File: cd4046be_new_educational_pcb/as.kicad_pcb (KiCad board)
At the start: 2 copper layers, 43.5 x 29.5 mm, 9 parts, among them IC1 CD4046BE, J1 Conn_01x02_Socket, J2 Conn_01x08_Socket, J3 Conn_01x08_Socket, J4 Conn_01x02_Socket, J5 Conn_01x02_Socket, J6 Conn_01x02_Socket, J7 Conn_01x02_Socket, J8 Conn_01x02_Socket

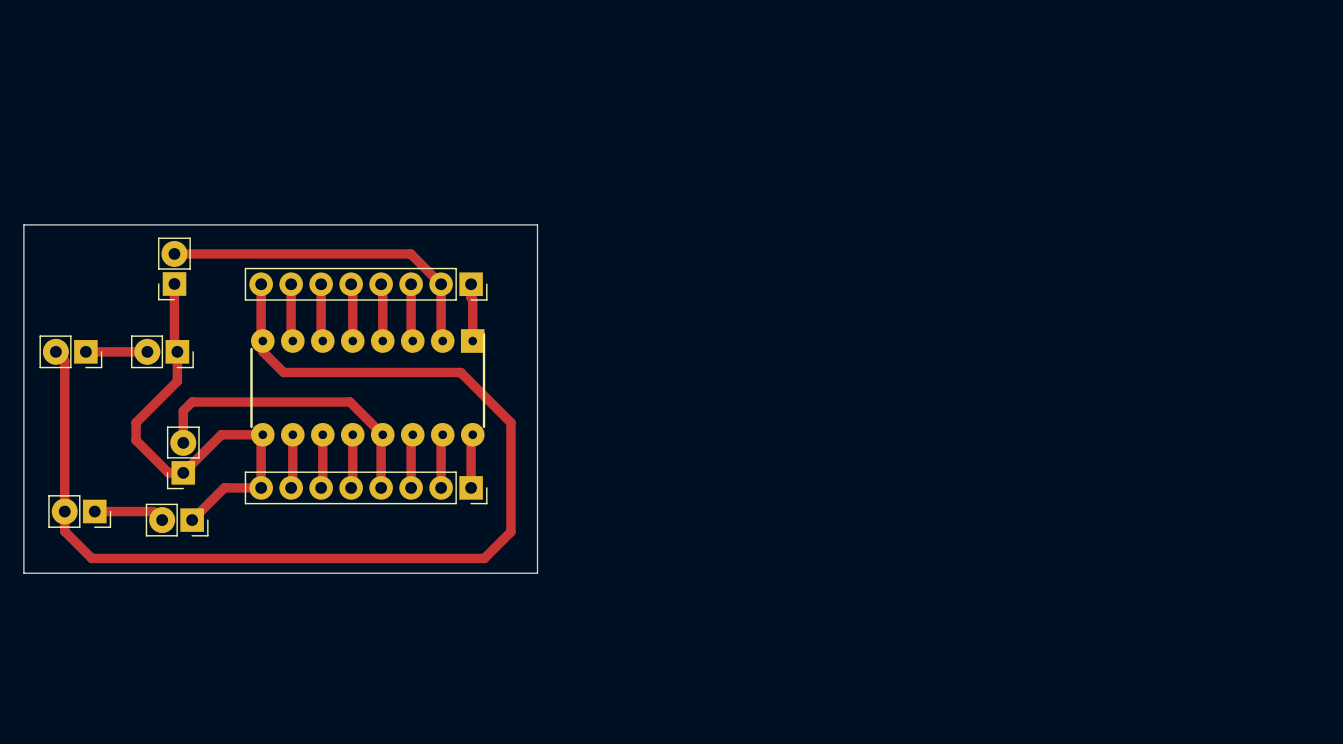
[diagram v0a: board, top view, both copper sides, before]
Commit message: a
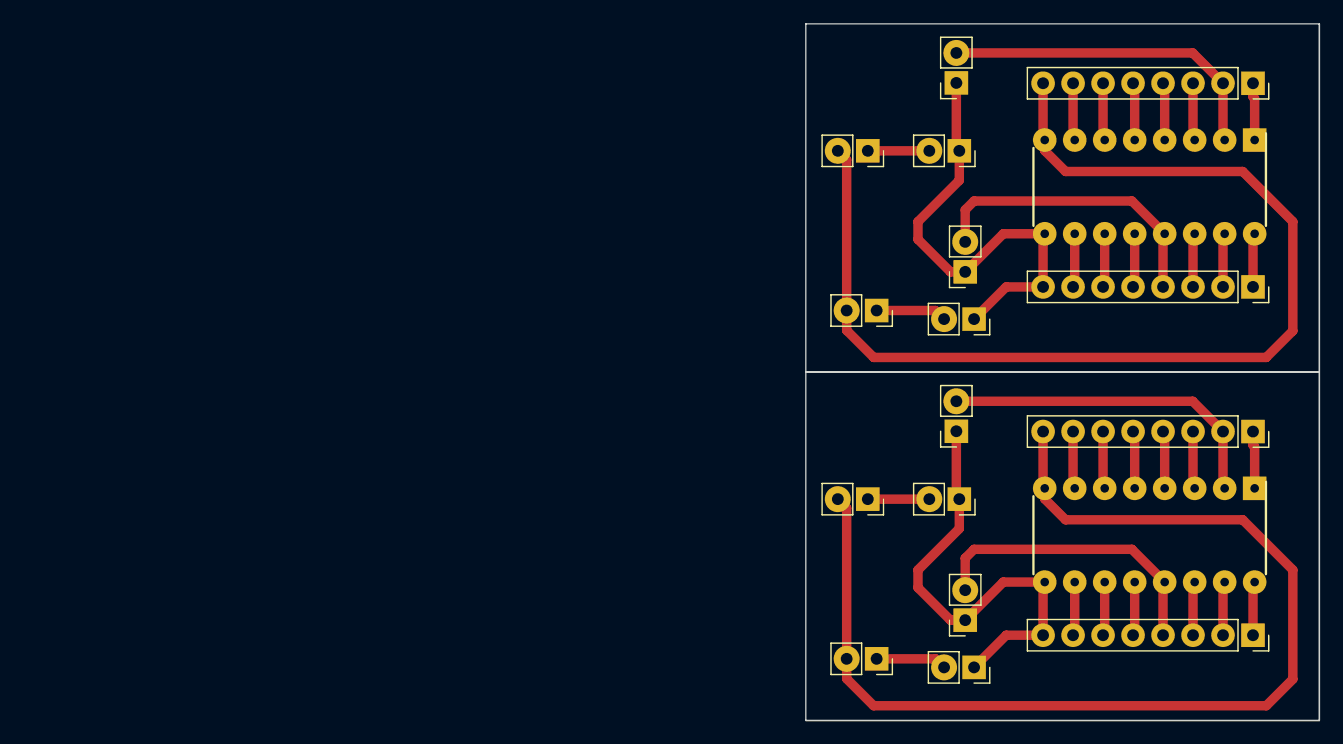
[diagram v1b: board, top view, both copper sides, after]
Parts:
- added IC1: CD4046BE, KiCad:DIP794W53P254L1930H508Q16N, F.Cu at (220.3, 107.5)
- added J1: Conn_01x02_Socket, Connector_PinSocket_2.54mm:PinSocket_1x02_P2.54mm_Vertical, F.Cu at (204.0, 98.7)
- added J2: Conn_01x08_Socket, Connector_PinSocket_2.54mm:PinSocket_1x08_P2.54mm_Vertical, F.Cu at (229.1, 98.8)
- added J3: Conn_01x08_Socket, Connector_PinSocket_2.54mm:PinSocket_1x08_P2.54mm_Vertical, F.Cu at (229.1, 116.0)
- added J4: Conn_01x02_Socket, Connector_PinSocket_2.54mm:PinSocket_1x02_P2.54mm_Vertical, F.Cu at (204.2, 104.5)
- added J5: Conn_01x02_Socket, Connector_PinSocket_2.54mm:PinSocket_1x02_P2.54mm_Vertical, F.Cu at (196.5, 104.5)
- added J6: Conn_01x02_Socket, Connector_PinSocket_2.54mm:PinSocket_1x02_P2.54mm_Vertical, F.Cu at (204.7, 114.7)
- added J7: Conn_01x02_Socket, Connector_PinSocket_2.54mm:PinSocket_1x02_P2.54mm_Vertical, F.Cu at (197.2, 118.0)
- added J8: Conn_01x02_Socket, Connector_PinSocket_2.54mm:PinSocket_1x02_P2.54mm_Vertical, F.Cu at (205.5, 118.7)
- moved IC1 68.4 mm to (220.3, 78.0)
- moved J1 68.4 mm to (204.0, 69.2)
- moved J2 68.4 mm to (229.1, 69.2)
- moved J3 68.4 mm to (229.1, 86.5)
- moved J4 68.4 mm to (204.2, 75.0)
- moved J5 68.4 mm to (196.5, 75.0)
- moved J6 68.4 mm to (204.7, 85.2)
- moved J7 68.4 mm to (197.2, 88.5)
- moved J8 68.4 mm to (205.5, 89.2)
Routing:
- net GND: track 93.7 -> 187.4 mm
- net /VCO_IN: track 40.7 -> 81.4 mm
- net /PC1: track 28.5 -> 57.0 mm
- net /PC2: track 25.6 -> 51.2 mm
- net Net-(J7-Pin_1): track 6.01 -> 12.0 mm
- net Net-(J4-Pin_2): track 5.21 -> 10.4 mm
- net Net-(IC1-PHASE_PULSES): track 4.87 -> 9.74 mm
- net Net-(IC1-INHIBIT): track 4.87 -> 9.74 mm
- net Net-(IC1-VCO_OUT): track 4.87 -> 9.74 mm
- net Net-(IC1-CI(1)): track 4.87 -> 9.74 mm
- net Net-(IC1-COMPARATOR_IN): track 4.87 -> 9.74 mm
- net Net-(IC1-CI(2)): track 4.87 -> 9.74 mm
- net VDD: track 4.56 -> 9.12 mm
- net Net-(IC1-R2_TO_VSS): track 4.56 -> 9.12 mm
- net Net-(IC1-ZENER): track 4.56 -> 9.12 mm
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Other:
- board size 43.5 x 29.5 mm -> 43.5 x 59 mm
